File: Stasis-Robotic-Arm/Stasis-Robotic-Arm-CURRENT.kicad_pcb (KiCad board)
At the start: 2 copper layers, 79 parts, among them J1 Screw_Terminal_01x04, J2 USB_C_Receptacle_USB2.0_14P, J3 Screw_Terminal_01x04, J4 Screw_Terminal_01x04, J5 Screw_Terminal_01x04, J6 Screw_Terminal_01x04, J7 Screw_Terminal_01x02, J8 Screw_Terminal_01x03, SW1 Enable, SW2 boot, U10 TVS1400DRV, U4 NCP1117-3.3_SOT223, U8 NCP1117-3.3_SOT223, U9 TVS1400DRV

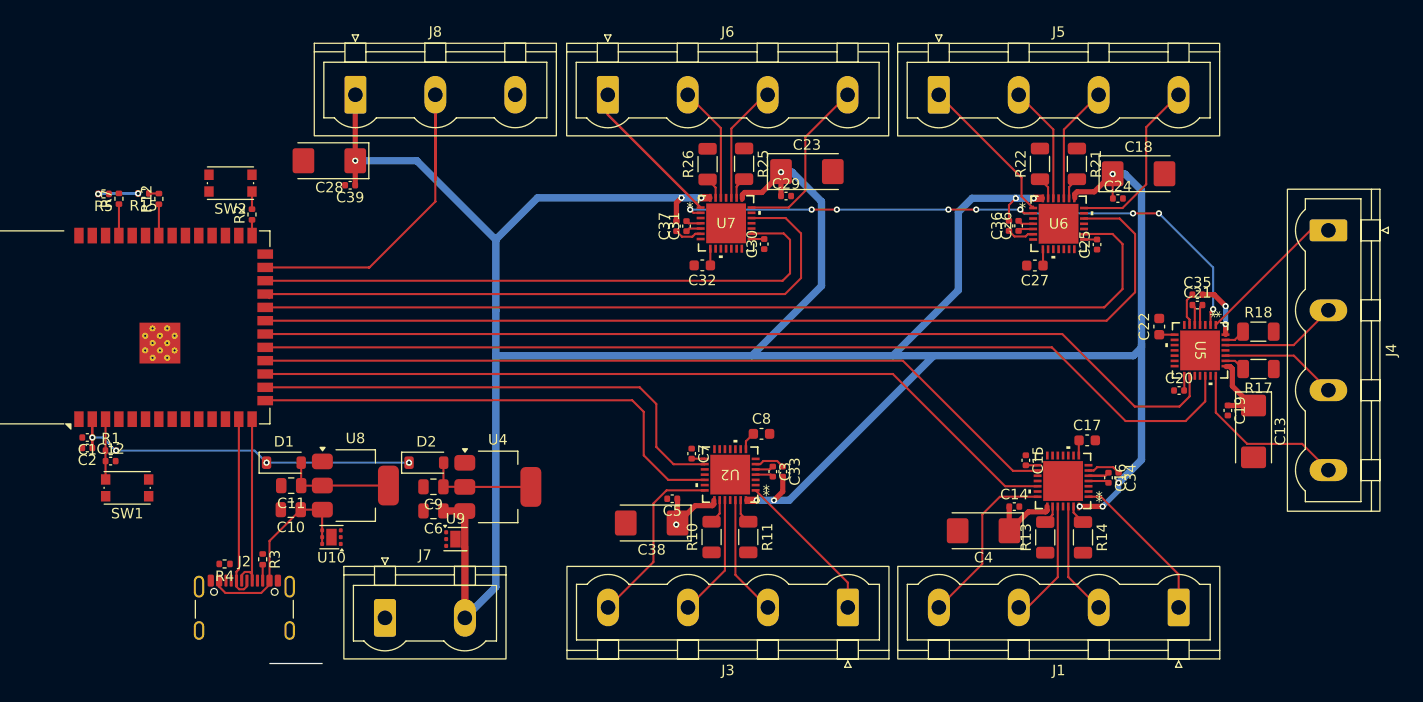
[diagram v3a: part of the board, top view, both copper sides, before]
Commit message: Add files via upload
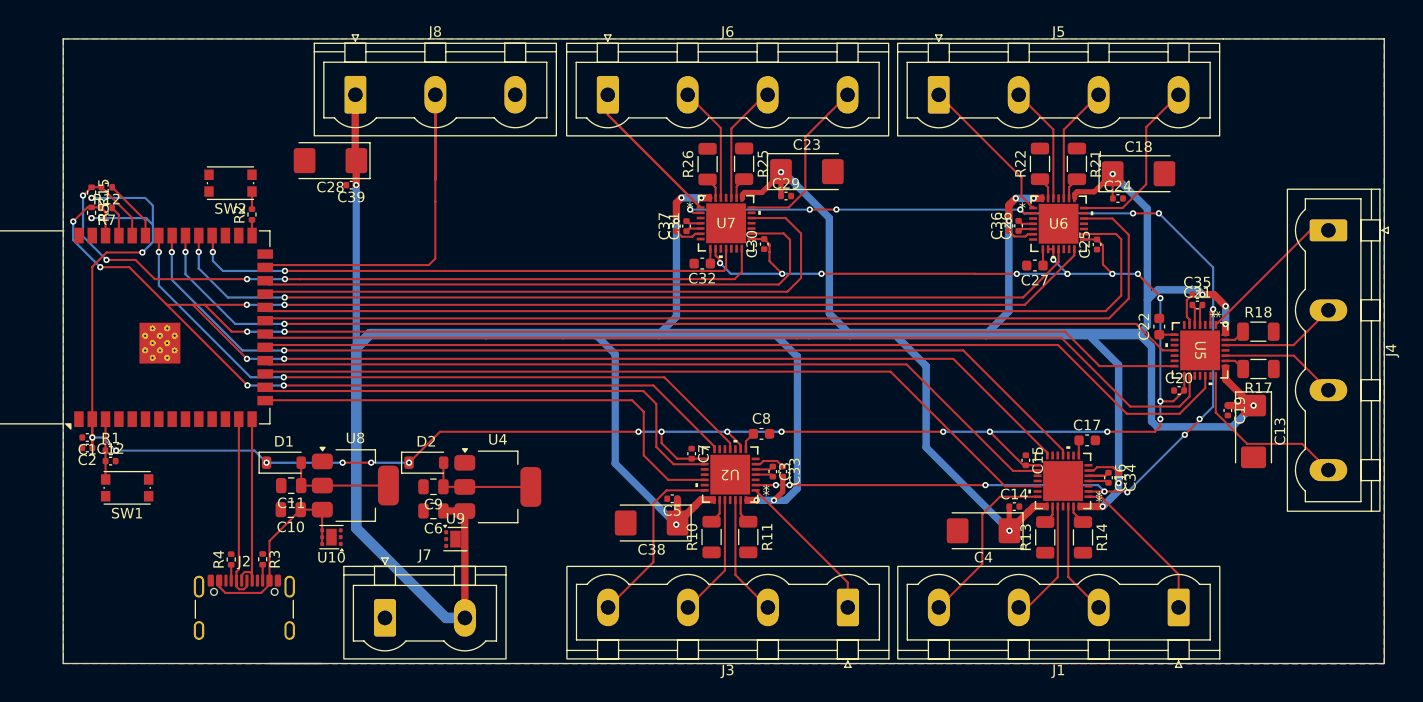
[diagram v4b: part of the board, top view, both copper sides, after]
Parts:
- moved R12 5.08 mm to (47.7, 117.4), turned to 180 degrees
- moved R15 4.95 mm to (46.2, 117.9), turned to -90 degrees
- moved R5 2.13 mm to (46.2, 119.8), turned to -90 degrees
- moved R7 1.46 mm to (47.6, 119.4), turned to 180 degrees
- moved R4 0.76 mm to (59.5, 152.9), turned to 90 degrees
- moved C32 0.17 mm to (104.4, 124.7)
- moved C39 0.11 mm to (71.0, 117.2)
- moved C28 0.11 mm to (69.0, 114.9)
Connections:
- U1 pad 30: /DIAG_1 -> /DIAG_5
- U1 pad 31: /DIAG_2 -> /DIAG_4
- U1 pad 33: /DIAG_4 -> /DIAG_2
- U1 pad 34: /DIAG_5 -> /DIAG_1
- U1 pad 36: /PDN-UART0 -> /PDN-UART1
- U1 pad 38: /PDN-UART1 -> /PDN-UART0
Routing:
- net /PDN-UART0: track 0.00 -> 349.1 mm, vias 0 -> 10
- net +3V3: track 50.8 -> 236.0 mm, vias 6 -> 27
- net /DIAG_3: track 0.00 -> 101.0 mm, vias 0 -> 2
- net /DIAG_2: track 0.00 -> 96.4 mm, vias 0 -> 2
- net /DIAG_4: track 0.00 -> 88.9 mm, vias 0 -> 2
- net /PDN-UART1: track 0.96 -> 78.9 mm, vias 0 -> 4
- net /DIAG_1: track 0.00 -> 66.0 mm, vias 0 -> 2
- net /ENN: track 60.2 -> 118.4 mm, vias 9 -> 14
- net /DIAG_5: track 0.00 -> 53.8 mm, vias 0 -> 2
- net VBAT: track 315.5 -> 365.7 mm, vias 15 -> 19
- net /TXD1: track 3.00 -> 6.27 mm
- net /PWM: track 37.2 -> 40.3 mm
- net Net-(J2-CC1): track 0.00 -> 1.51 mm
- net /DIR_3: track 95.7 -> 94.6 mm
- net /DIR_4: track 95.1 -> 94.2 mm
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- added copper zone on F.Cu, net GND
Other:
- board outline added: 125.9 x 59.6 mm
